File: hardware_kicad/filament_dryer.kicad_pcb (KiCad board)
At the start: 2 copper layers, 94 x 130 mm, 64 parts, among them J2 H/T Ambient, J3 T Aux, J4 Peristaltic Pump, U1 Pico, U4 DS18B20Z, U5 H/T Filament

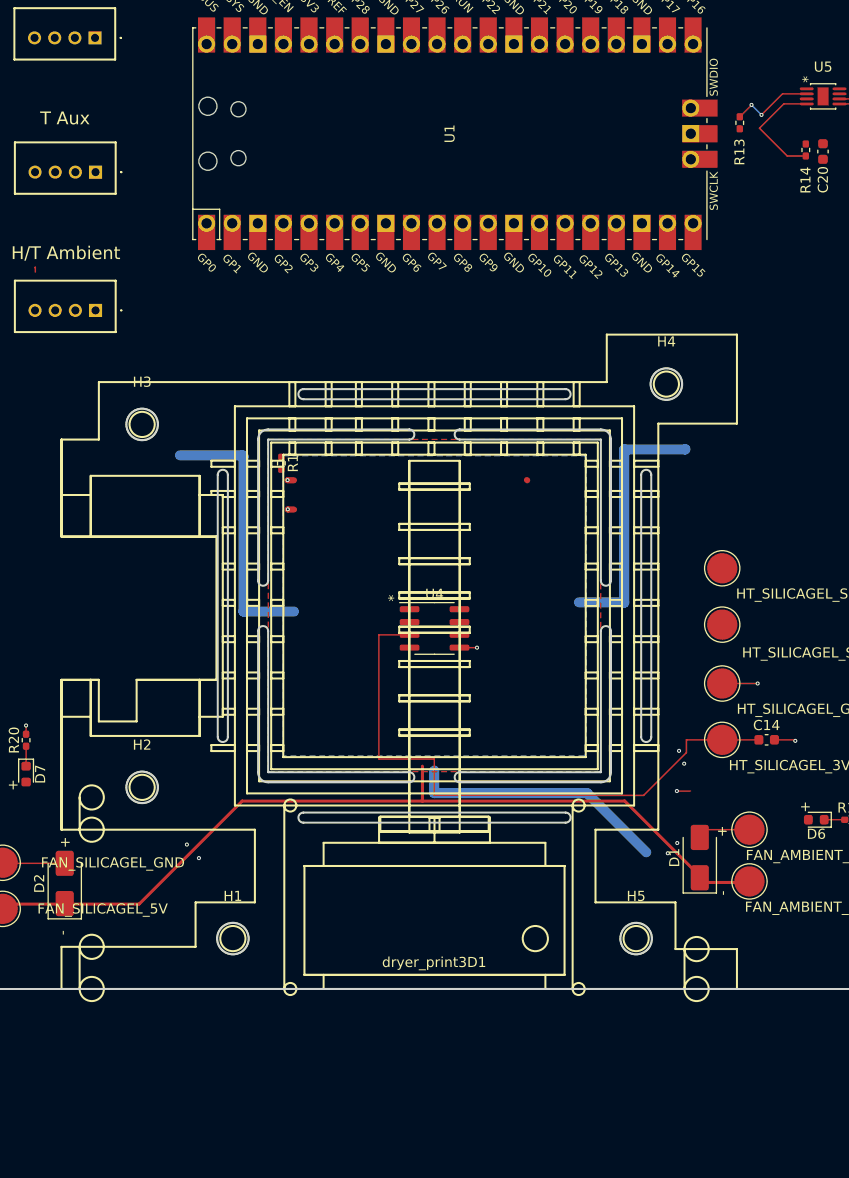
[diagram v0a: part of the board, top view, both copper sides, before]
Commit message: 20230917p_filament_dryer_silicagel.FCStd
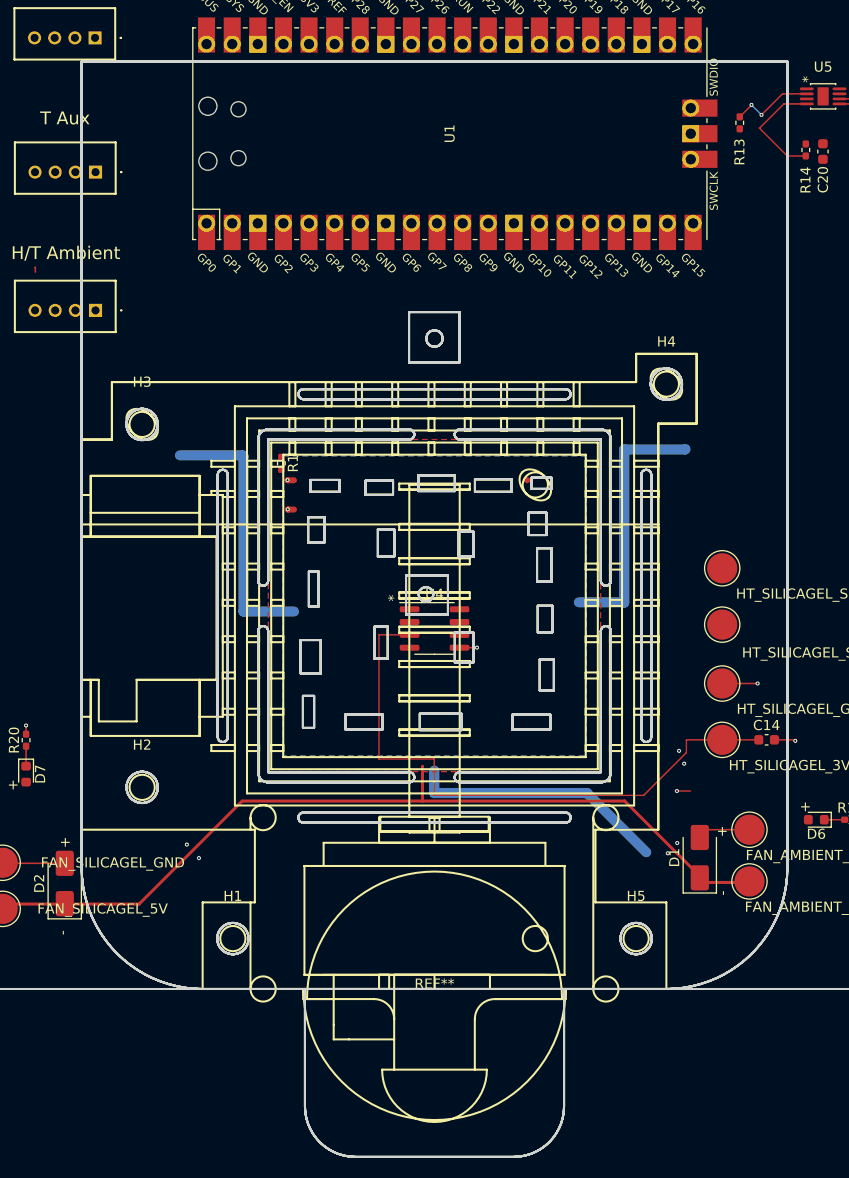
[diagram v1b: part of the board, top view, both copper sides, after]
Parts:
- removed dryer_print3D1: dryer_print3D, 00_project_library:dryer_print3d
- added REF**: dryer_print3d, 00_project_library:dryer_print3d, F.Cu at (101.0, 170.0)
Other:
- board size 94 x 130 mm -> 94 x 146.7 mm
